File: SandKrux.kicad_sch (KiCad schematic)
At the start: 119 parts, among them CN2 1.25mm-2P socket, IC1 TROPIC01_chip, Q1 S8050, SW1 TL3330AF130QG, SW2 TL3330AF130QG, SW3 TL3330AF130QG, SW4 TL3330AF130QG, SW5 TL3330AF130QG, U10 AXP173_C3345106, U11 GD32F150G8U6, U2 MT9700, U3 XC6206-3.3V, U9 HX TF-CARD XG8P H1.5, X2 X322526MMB4SI

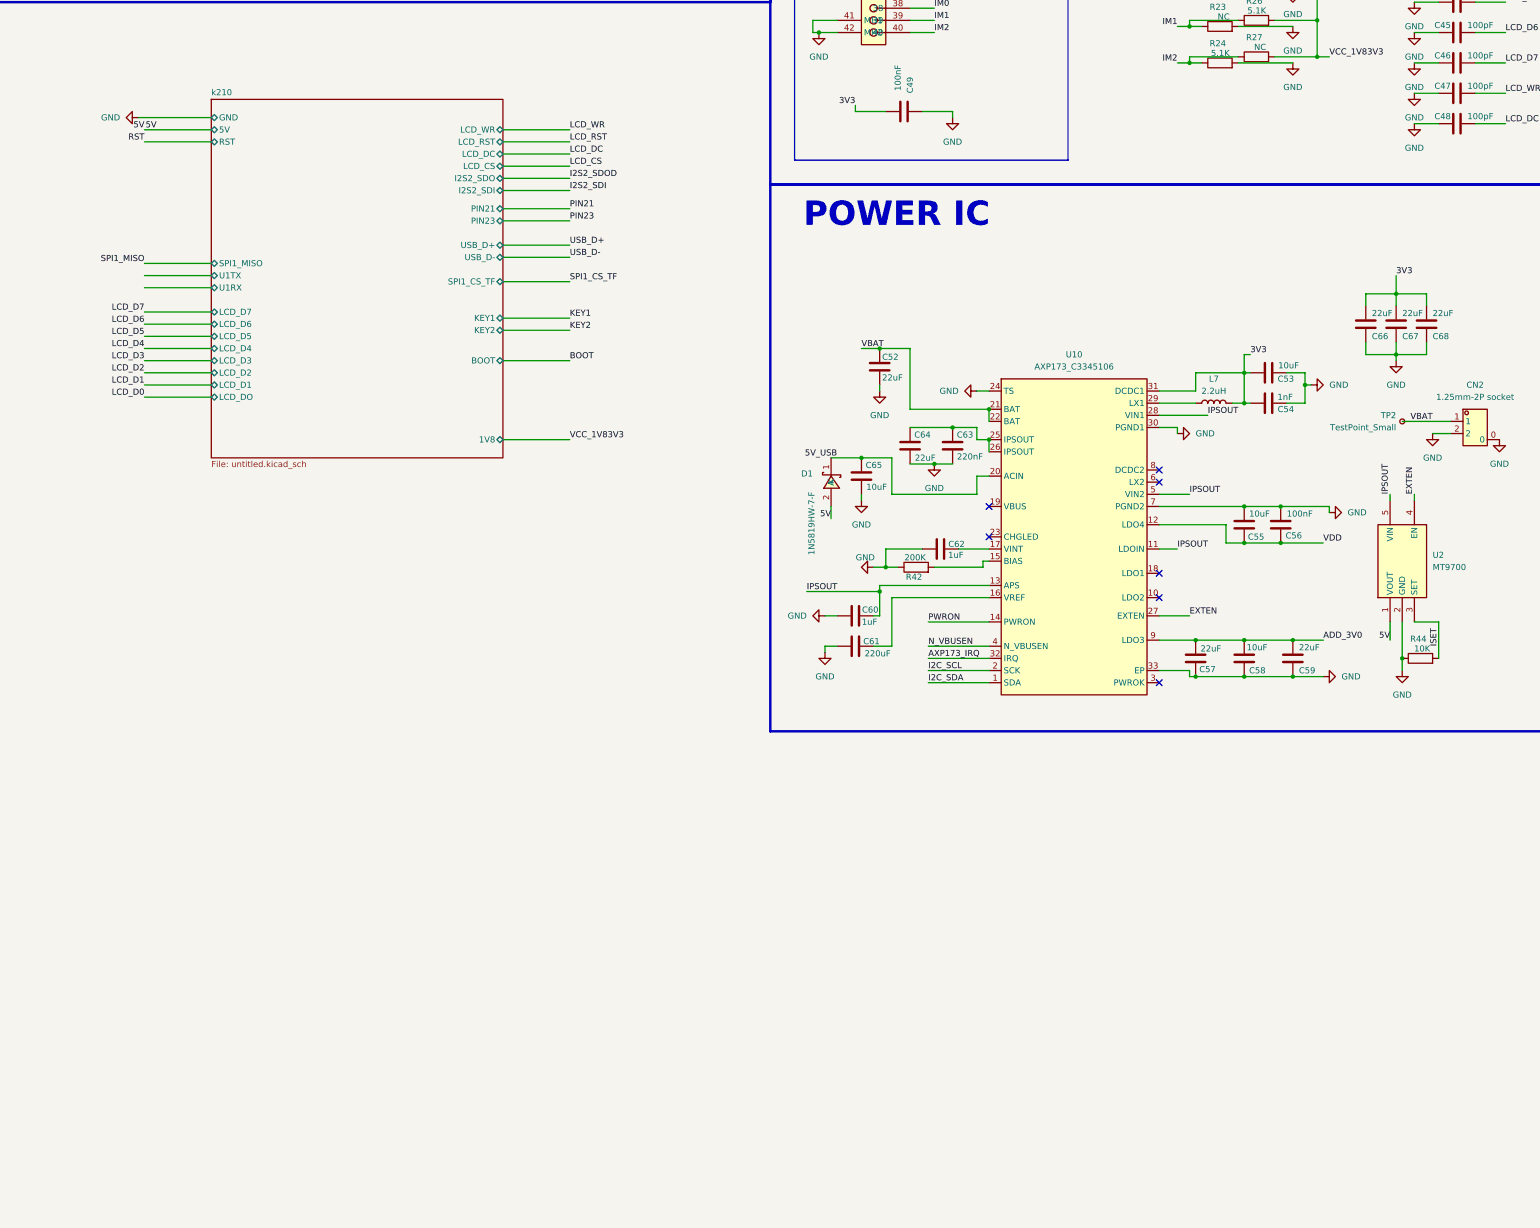
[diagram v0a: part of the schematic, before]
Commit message: ch340
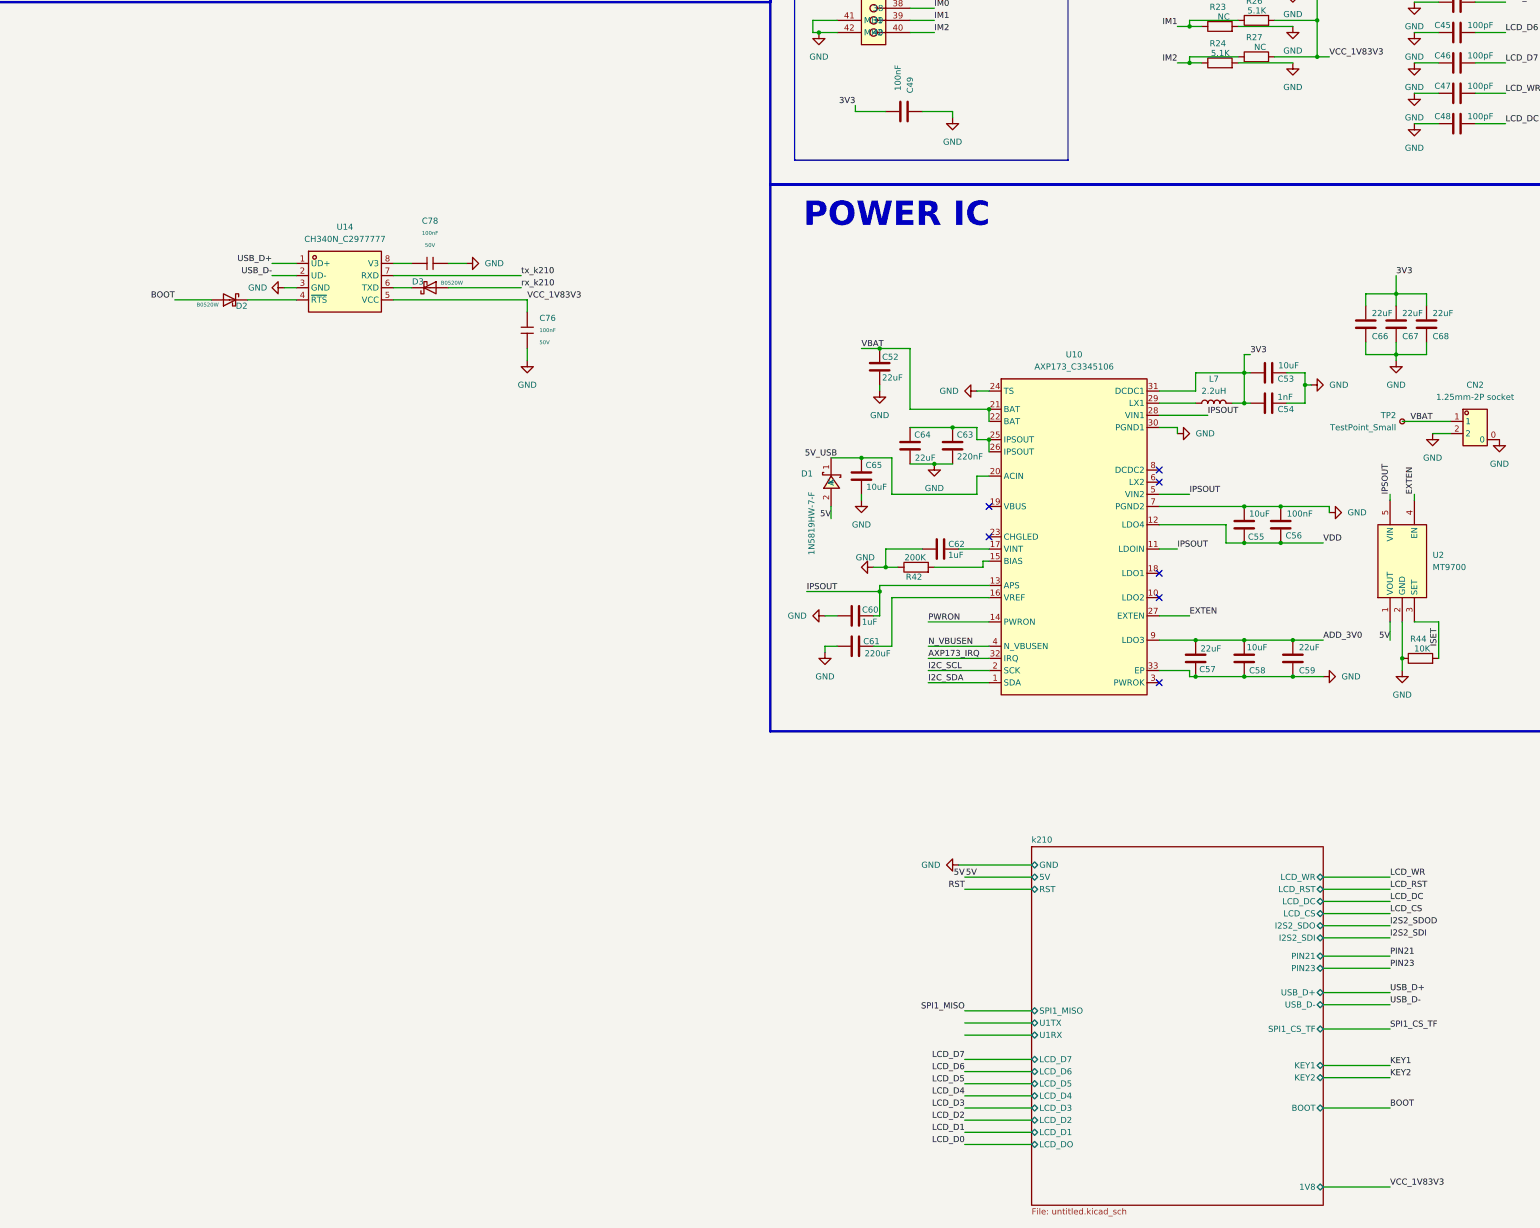
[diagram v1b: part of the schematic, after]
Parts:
- added C76, C78: 100nF, PCM_JLCPCB:C_0603, symbol PCM_JLCPCB-Capacitors:0603,100nF
- added D2, D3: B0520W, PCM_JLCPCB:D_SOD-123, symbol PCM_JLCPCB-Diodes:Schottky,B0520W
- added U14: CH340N_C2977777, easyeda2kicad:SOP-8_L4.9-W3.9-P1.27-LS6.0-BL, symbol easyeda2kicad:CH340N_C2977777
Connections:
- net BOOT: now also D2.2
- net GND: now also C76.2, C78.2, U14.3 (GND)
- net USB_D+: now also U14.1 (UD+)
- net USB_D-: now also U14.2 (UD-)
- net VCC_1V83V3: now also C76.1, U14.5 (VCC)
- new net: D3.1, U14.6 (TXD)
- new net: C78.1, U14.8 (V3)
- new net: D2.1, U14.4 (~{RTS})
- new net rx_k210: D3.2
- new net tx_k210: U14.7 (RXD)
